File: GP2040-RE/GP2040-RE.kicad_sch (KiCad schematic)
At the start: 57 parts, among them J1 I2C Target, J2 CONN HEADER R/A 6POS 2.54MM, J3 SM03B-SRSS-TB_LF__SN_, J4 GSB1C4621DS2HR, J5 Conn_01x03, J6 microSD, J7 RJ-45, J8 Conn_01x10, J9 Conn_01x02, U1 RP2040, U2 16M, U3 TXB0108PWR, U4 Linear Regulator

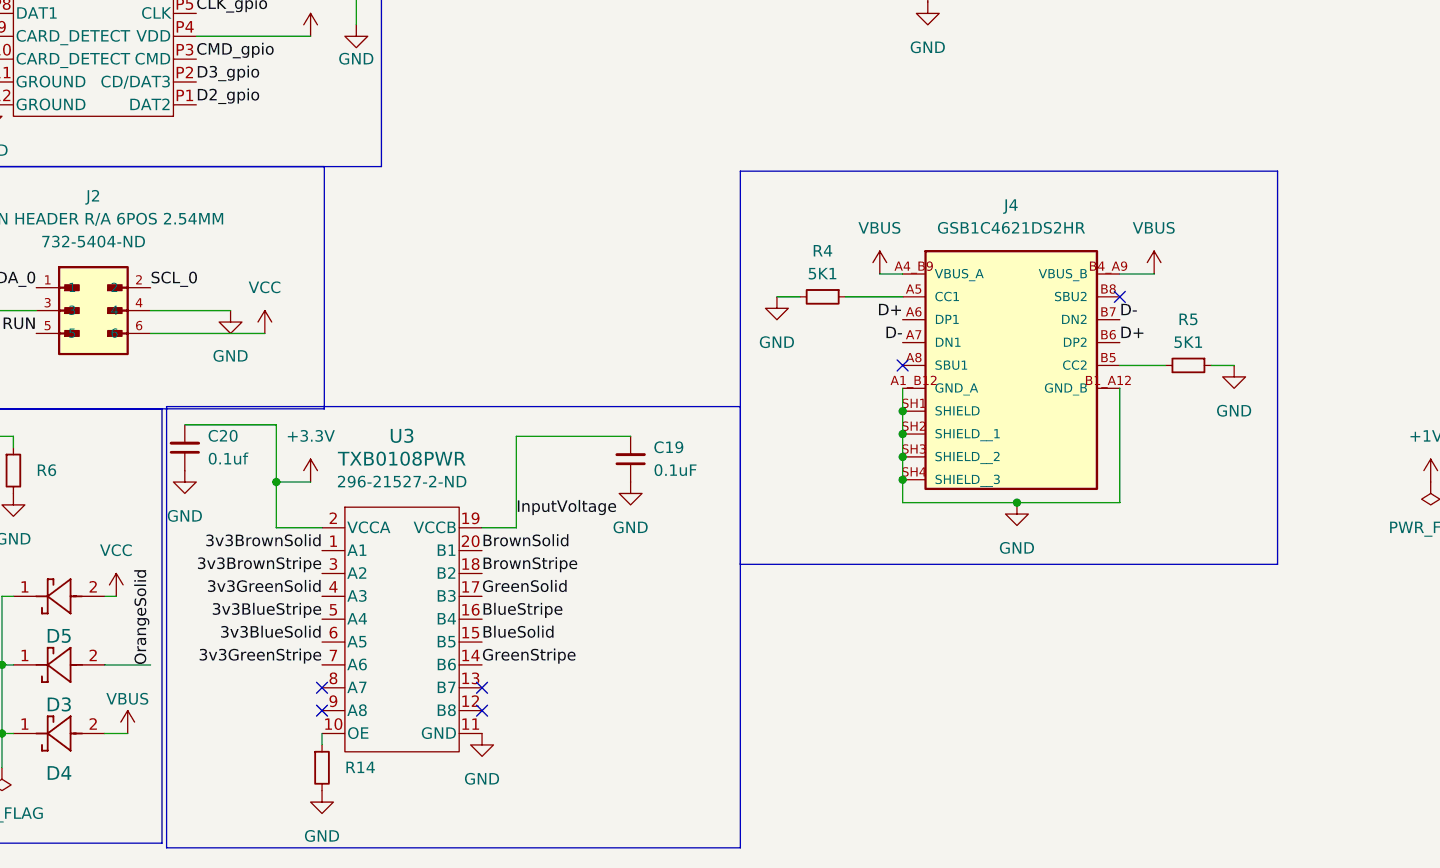
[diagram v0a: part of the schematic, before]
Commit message: Documentation day
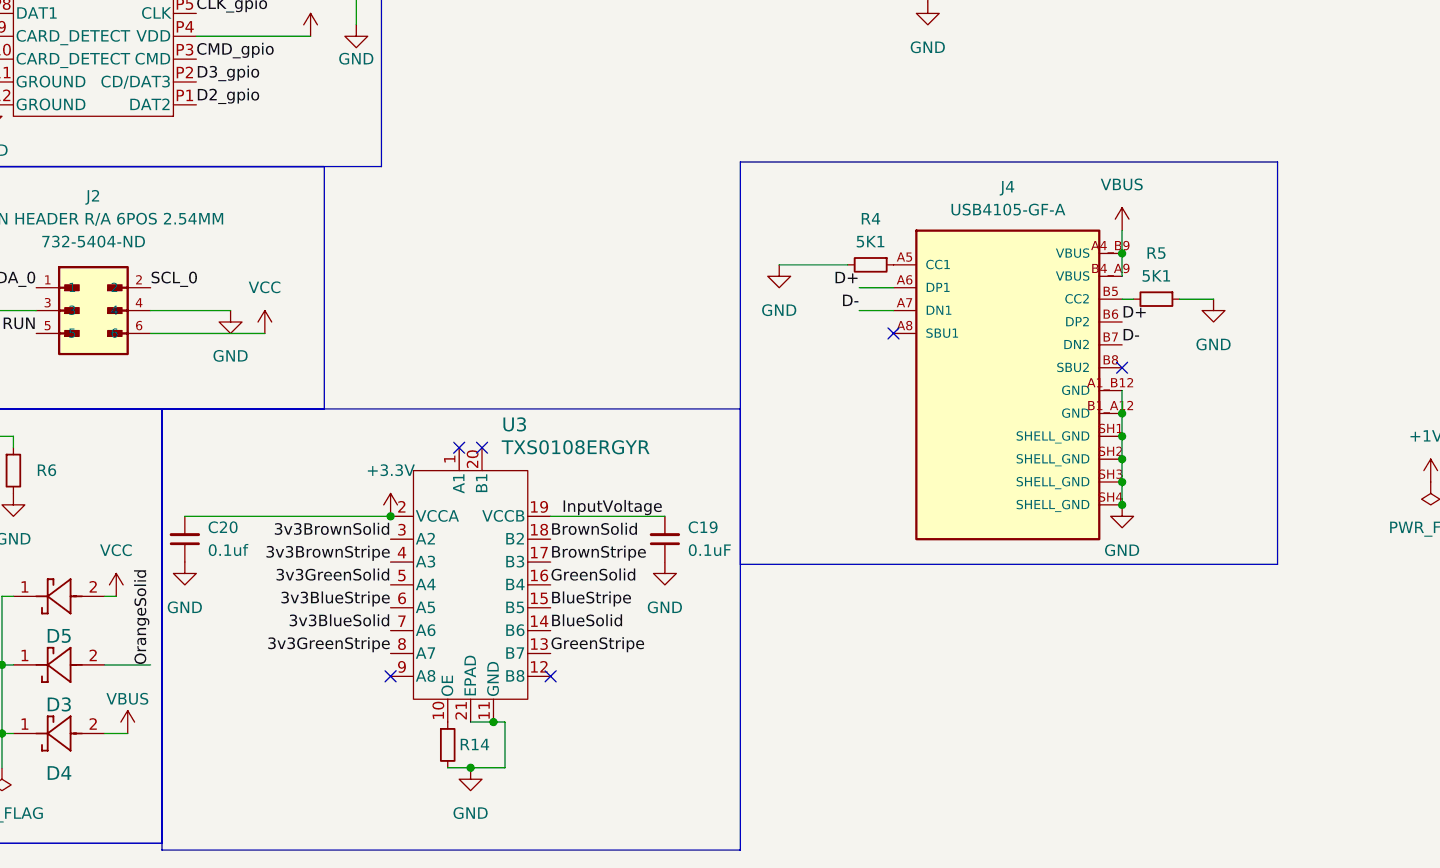
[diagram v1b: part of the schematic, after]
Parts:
- removed U3: TXB0108PWR, GP2040-RE:TXB0108PWR, symbol GP2040-RE:TXB0108PWR
- added U3: TXS0108ERGYR, GP2040-RE:RGY20_3P05X2P05, symbol GP2040-RE:TXS0108ERGYR
- J4: value GSB1C4621DS2HR -> USB4105-GF-A; footprint GP2040-RE:AMPHENOL_GSB1C4621DS2HR -> GP2040-RE:GCT_USB4105-GF-A; symbol GP2040-RE:GSB1C4621DS2HR -> GP2040-RE:USB4105-GF-A; DigiKey Part Number 664-GSB1C4621DS2HRCT-ND -> 2073-USB4105-GF-ACT-ND
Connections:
- net +3.3V: now also U3.2 (VCCA)
- net 3v3BlueSolid: now also U3.7 (A6)
- net 3v3BlueStripe: now also U3.6 (A5)
- net 3v3BrownSolid: now also U3.3 (A2)
- net 3v3BrownStripe: now also U3.4 (A3)
- net 3v3GreenSolid: now also U3.5 (A4)
- net 3v3GreenStripe: now also U3.8 (A7)
- net BlueSolid: now also U3.14 (B6)
- net BlueStripe: now also U3.15 (B5)
- net BrownSolid: now also U3.18 (B2)
- net BrownStripe: now also U3.17 (B3)
- net GND: now also U3.11 (GND), U3.21 (EPAD)
- net GreenSolid: now also U3.16 (B4)
- net GreenStripe: now also U3.13 (B7)
- net InputVoltage: now also U3.19 (VCCB)
- net at R14.1: now also U3.10 (OE)
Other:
- moved on the sheet: C19, C20, J4, R14, R4, R5
